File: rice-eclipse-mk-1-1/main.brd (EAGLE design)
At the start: 110.2 x 91.2 mm, 106 parts, among them IC1 LMV321LICTRT, IC2 LMV321LICTRT, IC3 LMV321LICTRT, IC4 LMV321LICTRT, IC5 UA78M, IC6 LMV321LICTRT, U1 LM1084ISX-5.0/NOPB, U2 THS4531IDRD8-M, U3 THS4531IDRD8-M, U4 THS4531IDRD8-M, U5 THS4531IDRD8-M, U6 1101M2S3CQE2, X1 2540-5

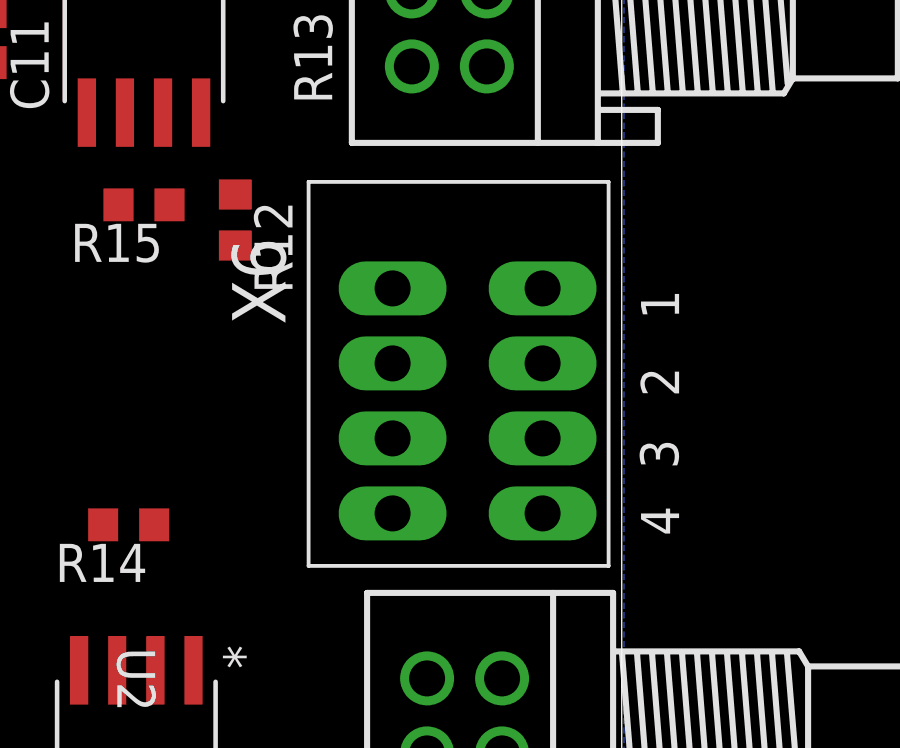
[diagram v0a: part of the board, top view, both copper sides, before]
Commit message: Added some stuff.
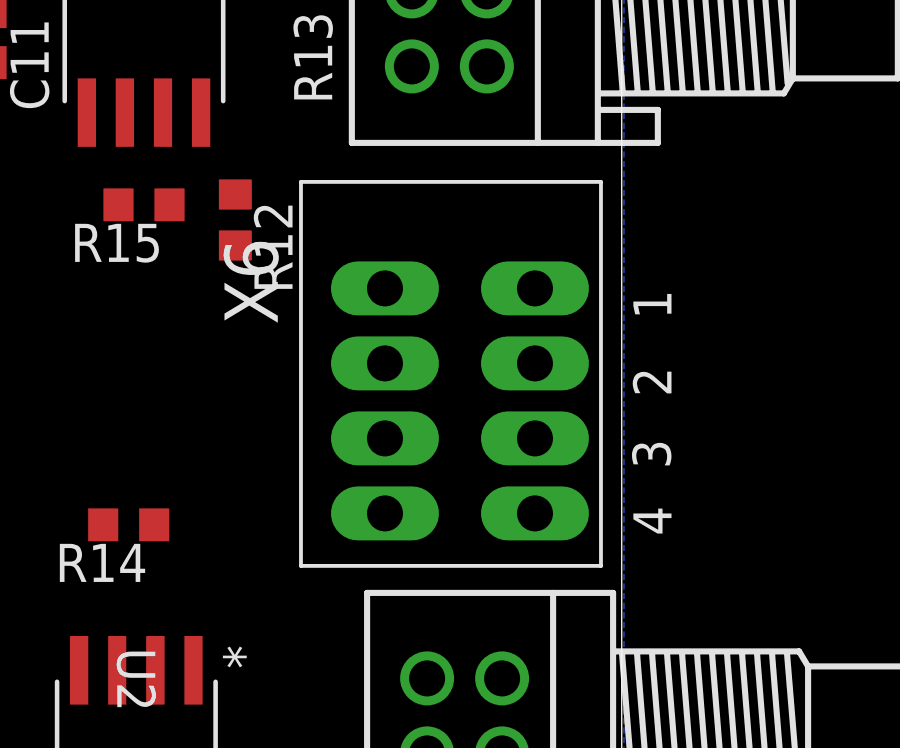
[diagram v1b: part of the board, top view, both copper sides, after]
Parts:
- moved X6 0.25 mm to (99.6, 40.9)
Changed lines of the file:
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@@
 <element name="R25" library="rcl" library_urn="urn:adsk.eagle:library:334" package="R0603" package3d_urn="urn:adsk.eagle:package:23555/2" value="500K" x="59.436" y="81.28" rot="R180"/>
 <element name="X5" library="con-phoenix-250-extra" package="1770908" value="" x="99.568" y="77.978" rot="R270"/>
-<element name="X6" library="con-phoenix-250-extra" package="1770908" value="" x="99.822" y="40.894" rot="R270"/>
+<element name="X6" library="con-phoenix-250-extra" package="1770908" value="" x="99.568" y="40.894" rot="R270"/>
 <element name="U6" library="SLIDE_SW" package="1101M2S3CQE2" value="1101M2S3CQE2" x="26.67" y="2.794">
 <attribute name="COPYRIGHT" value="Copyright (C) 2015 Accelerated Designs. All rights reserved" x="26.67" y="2.794" size="1.778" layer="27" display="off"/>
@@
 <contactref element="X6" pad="P$8"/>
 <contactref element="X6" pad="P$4"/>
-<wire x1="102.522" y1="29.844" x2="107.522" y2="29.844" width="0" layer="19" extent="1-1"/>
-<wire x1="106.172" y1="21.844" x2="107.522" y2="29.844" width="0" layer="19" extent="1-1"/>
+<wire x1="102.268" y1="29.844" x2="107.268" y2="29.844" width="0" layer="19" extent="1-1"/>
+<wire x1="106.172" y1="21.844" x2="107.268" y2="29.844" width="0" layer="19" extent="1-1"/>
 </signal>
 <signal name="LC_1_OUT+">
@@
 <contactref element="X6" pad="P$3"/>
 <contactref element="X6" pad="P$7"/>
-<wire x1="102.522" y1="32.344" x2="107.522" y2="32.344" width="0" layer="19" extent="1-1"/>
-<wire x1="103.672" y1="21.844" x2="102.522" y2="32.344" width="0" layer="19" extent="1-1"/>
+<wire x1="102.268" y1="32.344" x2="107.268" y2="32.344" width="0" layer="19" extent="1-1"/>
+<wire x1="103.672" y1="21.844" x2="102.268" y2="32.344" width="0" layer="19" extent="1-1"/>
 </signal>
 <signal name="ADC1_A0">
@@
 <contactref element="X6" pad="P$2"/>
 <contactref element="X6" pad="P$6"/>
-<wire x1="107.522" y1="34.844" x2="105.664" y2="47.244" width="0" layer="19" extent="1-1"/>
-<wire x1="102.522" y1="34.844" x2="107.522" y2="34.844" width="0" layer="19" extent="1-1"/>
+<wire x1="107.268" y1="34.844" x2="105.664" y2="47.244" width="0" layer="19" extent="1-1"/>
+<wire x1="102.268" y1="34.844" x2="107.268" y2="34.844" width="0" layer="19" extent="1-1"/>
 </signal>
 <signal name="LC_2_OUT+">
@@
 <contactref element="X6" pad="P$5"/>
 <contactref element="X6" pad="P$1"/>
-<wire x1="102.522" y1="37.344" x2="103.164" y2="47.244" width="0" layer="19" extent="1-1"/>
-<wire x1="107.522" y1="37.344" x2="102.522" y2="37.344" width="0" layer="19" extent="1-1"/>
+<wire x1="102.268" y1="37.344" x2="103.164" y2="47.244" width="0" layer="19" extent="1-1"/>
+<wire x1="107.268" y1="37.344" x2="102.268" y2="37.344" width="0" layer="19" extent="1-1"/>
 </signal>
 <signal name="ADC1_A2">
